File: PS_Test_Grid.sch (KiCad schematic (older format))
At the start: 50 parts, among them J1 CONN_01X03, J10 CONN_01X01, J2 CONN_01X01, J3 CONN_01X01, J4 CONN_01X01, J5 CONN_01X01, J6 CONN_01X03, J7 CONN_01X01, J8 CONN_01X01, J9 CONN_01X01, Q1 PhotoTransistor, U1 NOA1212, U2 MCP6001R, U3 MCP6001R

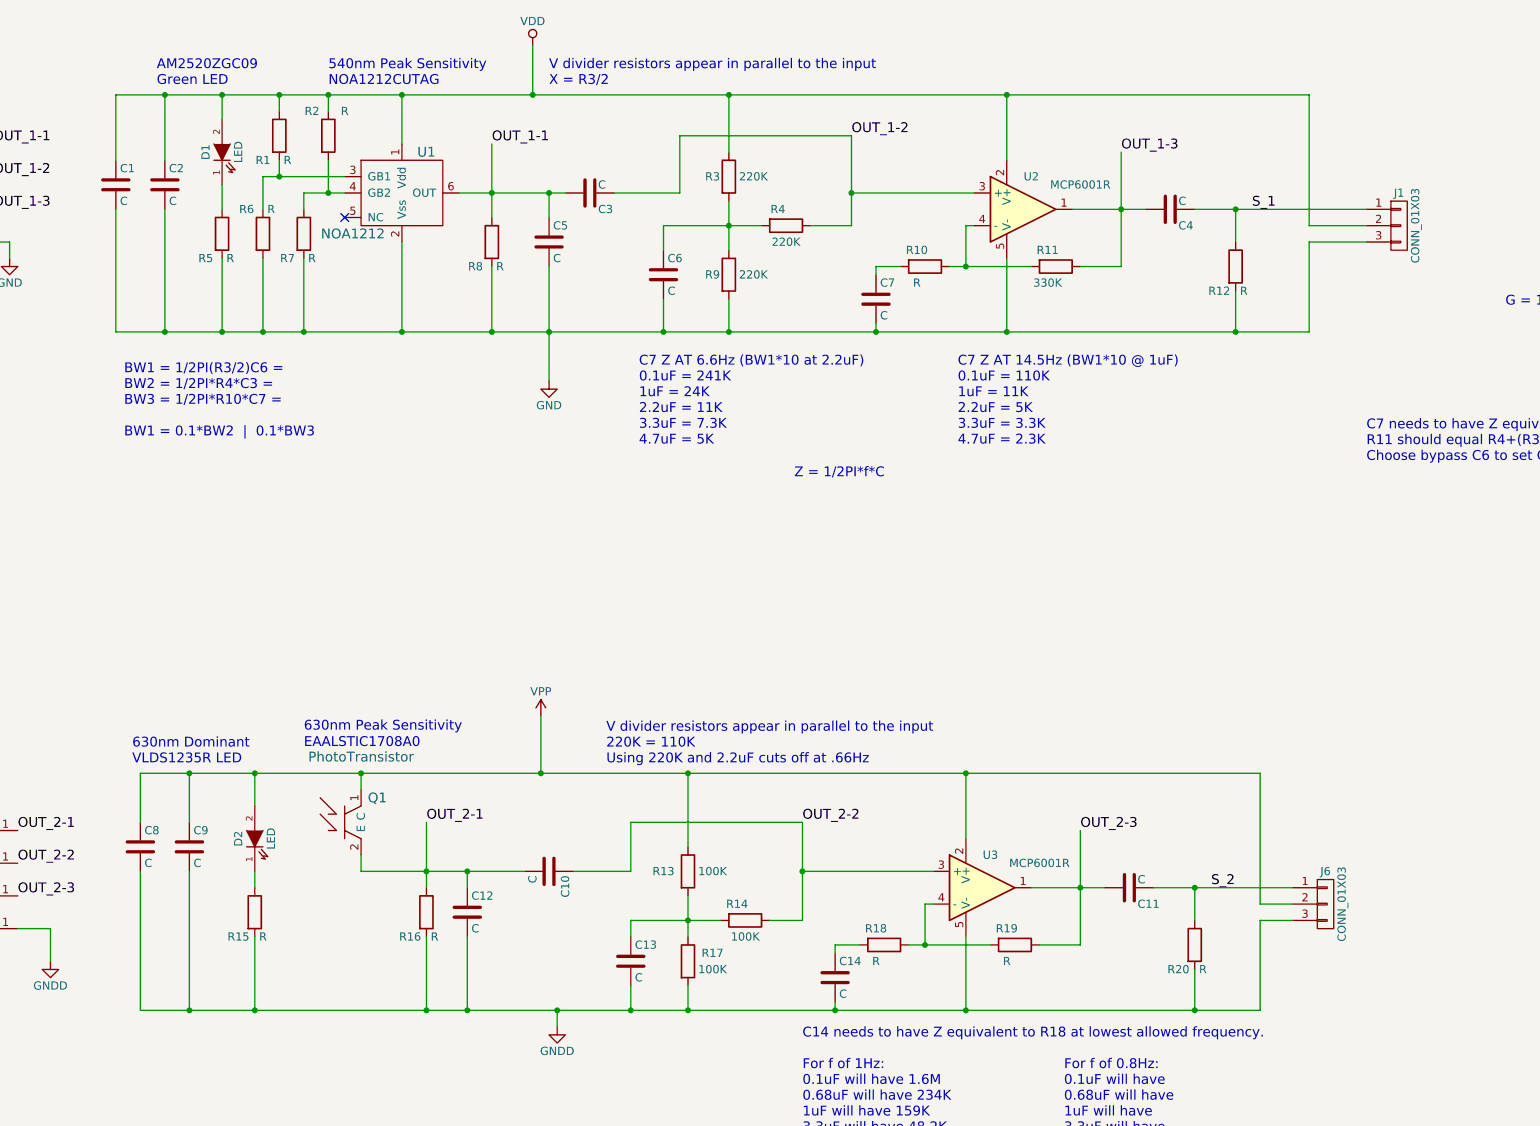
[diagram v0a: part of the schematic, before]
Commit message: saved notes
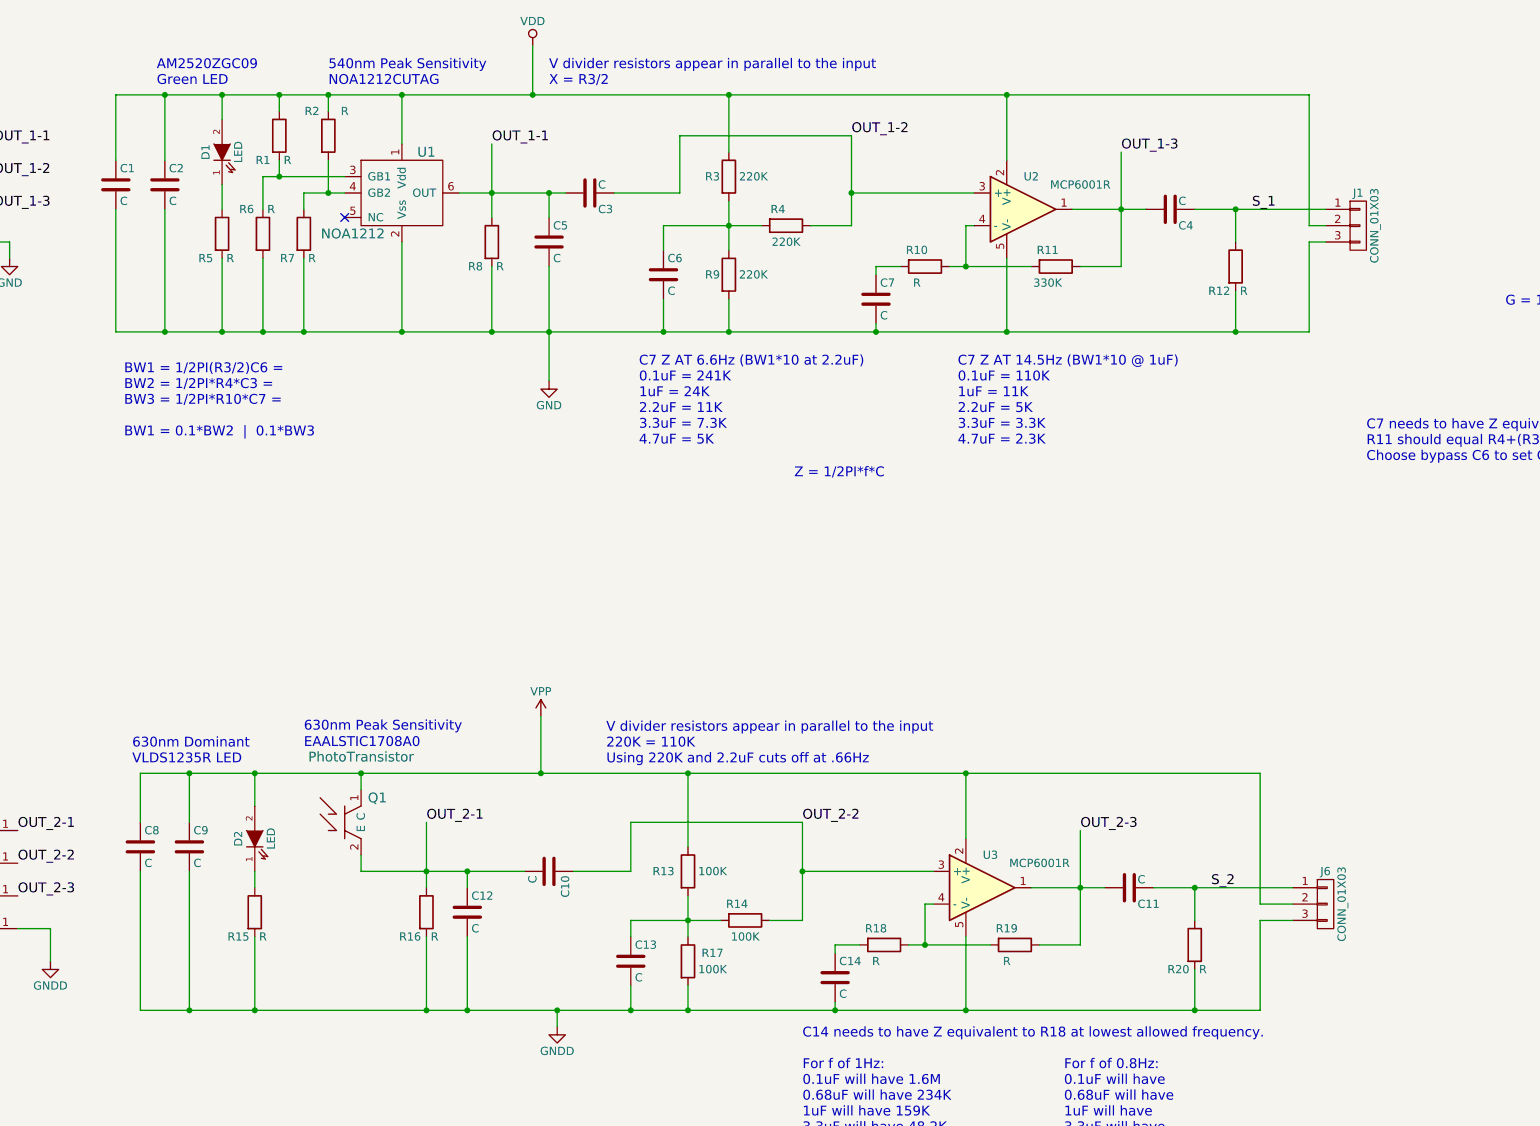
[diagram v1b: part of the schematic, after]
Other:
- moved on the sheet: J1
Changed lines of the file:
@@
 	7150 3550 7150 3000
 Wire Wire Line
-	8050 3150 8050 3850
+	8050 3150 8050 3550
+Wire Wire Line
+	8050 3550 8050 3850
 Wire Wire Line
 	10850 3550 10850 3100
@@
 	7150 2100 7150 2400
 Wire Wire Line
-	5400 2100 12700 2100
+	5400 2100 5700 2100
+Wire Wire Line
+	5700 2100 6050 2100
+Wire Wire Line
+	6050 2100 6400 2100
+Wire Wire Line
+	6400 2100 6700 2100
+Wire Wire Line
+	6700 2100 7150 2100
+Wire Wire Line
+	7150 2100 7950 2100
+Wire Wire Line
+	7950 2100 9150 2100
+Wire Wire Line
+	9150 2100 10850 2100
+Wire Wire Line
+	10850 2100 12700 2100
 Wire Wire Line
 	7950 2100 7950 1800
@@
 Connection ~ 7150 3550
 Wire Wire Line
-	7500 2700 8150 2700
-Wire Wire Line
-	7700 2400 7700 2850
+	7500 2700 7700 2700
+Wire Wire Line
+	7700 2700 8050 2700
+Wire Wire Line
+	8050 2700 8150 2700
+Wire Wire Line
+	7700 2400 7700 2700
+Wire Wire Line
+	7700 2700 7700 2850
 Wire Wire Line
 	7700 3550 7700 3150
@@
 Connection ~ 9150 2100
 Wire Wire Line
-	9150 2750 9150 3050
+	9150 2750 9150 2900
+Wire Wire Line
+	9150 2900 9150 3050
 Wire Wire Line
 	9150 3550 9150 3350
@@
 Connection ~ 9150 2900
 Wire Wire Line
-	11250 2800 11700 2800
-Wire Wire Line
-	11550 2450 11550 3150
+	11250 2800 11550 2800
+Wire Wire Line
+	11550 2800 11700 2800
+Wire Wire Line
+	11550 2450 11550 2800
+Wire Wire Line
+	11550 2800 11550 3150
 Wire Wire Line
 	11550 3150 11300 3150
@@
 	10600 2900 10600 3150
 Wire Wire Line
-	10500 3150 11000 3150
+	10500 3150 10600 3150
+Wire Wire Line
+	10600 3150 11000 3150
 Connection ~ 10600 3150
 Wire Wire Line
@@
 Connection ~ 6550 3550
 Wire Wire Line
-	6550 2700 6800 2700
+	6550 2700 6700 2700
+Wire Wire Line
+	6700 2700 6800 2700
 Wire Wire Line
 	6550 2700 6550 2800
@@
 Connection ~ 6700 2700
 Wire Wire Line
-	6300 2600 6800 2600
+	6300 2600 6400 2600
+Wire Wire Line
+	6400 2600 6800 2600
 Wire Wire Line
 	6300 2600 6300 2800
@@
 Connection ~ 7550 7700
 Wire Wire Line
-	6900 6850 7900 6850
+	6900 6850 7300 6850
+Wire Wire Line
+	7300 6850 7550 6850
+Wire Wire Line
+	7550 6850 7900 6850
 Wire Wire Line
 	7550 6850 7550 6950
@@
 Connection ~ 7550 6850
 Wire Wire Line
-	7300 6550 7300 6950
+	7300 6550 7300 6850
+Wire Wire Line
+	7300 6850 7300 6950
 Connection ~ 7300 6850
 Wire Wire Line
@@
 Connection ~ 11550 2800
 Wire Wire Line
-	12000 2800 13050 2800
+	12000 2800 12250 2800
+Wire Wire Line
+	12250 2800 12800 2800
 Wire Wire Line
 	12250 2800 12250 3000
@@
 Connection ~ 8900 6250
 Wire Wire Line
-	8900 7000 8900 7250
+	8900 7000 8900 7150
+Wire Wire Line
+	8900 7150 8900 7250
 Wire Wire Line
 	8900 7700 8900 7550
@@
 Connection ~ 8900 7150
 Wire Wire Line
-	11000 6950 11450 6950
-Wire Wire Line
-	11300 6600 11300 7300
+	11000 6950 11300 6950
+Wire Wire Line
+	11300 6950 11450 6950
+Wire Wire Line
+	11300 6600 11300 6950
+Wire Wire Line
+	11300 6950 11300 7300
 Wire Wire Line
 	11300 7300 11050 7300
@@
 	10350 7050 10350 7300
 Wire Wire Line
-	10250 7300 10750 7300
+	10250 7300 10350 7300
+Wire Wire Line
+	10350 7300 10750 7300
 Connection ~ 10350 7300
 Text Notes 8400 6200 0    60   ~ 0
@@
 Connection ~ 11300 6950
 Wire Wire Line
-	11750 6950 12600 6950
+	11750 6950 12000 6950
+Wire Wire Line
+	12000 6950 12600 6950
 Wire Wire Line
 	12000 6950 12000 7150
@@
 Connection ~ 5850 7700
 Wire Wire Line
-	5550 6250 12400 6250
-Wire Wire Line
-	5550 7700 12400 7700
+	5550 6250 5850 6250
+Wire Wire Line
+	5850 6250 6250 6250
+Wire Wire Line
+	6250 6250 6900 6250
+Wire Wire Line
+	6900 6250 8000 6250
+Wire Wire Line
+	8000 6250 8900 6250
+Wire Wire Line
+	8900 6250 10600 6250
+Wire Wire Line
+	10600 6250 12400 6250
+Wire Wire Line
+	5550 7700 5850 7700
+Wire Wire Line
+	5850 7700 6250 7700
+Wire Wire Line
+	6250 7700 7300 7700
+Wire Wire Line
+	7300 7700 7550 7700
+Wire Wire Line
+	7550 7700 8100 7700
+Wire Wire Line
+	8100 7700 8550 7700
+Wire Wire Line
+	8550 7700 8900 7700
+Wire Wire Line
+	8900 7700 9800 7700
+Wire Wire Line
+	9800 7700 10600 7700
+Wire Wire Line
+	10600 7700 12000 7700
+Wire Wire Line
+	12000 7700 12400 7700
 Connection ~ 10600 7700
 $Comp
@@
 L CONN_01X03 J1
 U 1 1 5B92B63C
-P 13250 2900
-F 0 "J1" H 13250 3100 50  0000 C CNN
-F 1 "CONN_01X03" V 13350 2900 50  0000 C CNN
-F 2 "Pin_Headers:Pin_Header_Straight_1x03_Pitch2.54mm" H 13250 2900 50  0001 C CNN
-F 3 "" H 13250 2900 50  0001 C CNN
-	1    13250 2900
+P 13000 2900
+F 0 "J1" H 13000 3100 50  0000 C CNN
+F 1 "CONN_01X03" V 13100 2900 50  0000 C CNN
+F 2 "Pin_Headers:Pin_Header_Straight_1x03_Pitch2.54mm" H 13000 2900 50  0001 C CNN
+F 3 "" H 13000 2900 50  0001 C CNN
+	1    13000 2900
 	1    0    0    -1
 $EndComp
@@
 	12400 6250 12400 7050
 Wire Wire Line
-	13050 2900 12700 2900
-Wire Wire Line
-	13050 3000 12700 3000
+	12800 2900 12700 2900
+Wire Wire Line
+	12800 3000 12700 3000
 Wire Wire Line
 	12700 3000 12700 3550
@@
 AM2520ZGC09\nGreen LED
 Wire Wire Line
-	12700 3550 5400 3550
+	12700 3550 12250 3550
+Wire Wire Line
+	12250 3550 10850 3550
+Wire Wire Line
+	10850 3550 10050 3550
+Wire Wire Line
+	10050 3550 9150 3550
+Wire Wire Line
+	9150 3550 8750 3550
+Wire Wire Line
+	8750 3550 8050 3550
+Wire Wire Line
+	8050 3550 7700 3550
+Wire Wire Line
+	7700 3550 7150 3550
+Wire Wire Line
+	7150 3550 6550 3550
+Wire Wire Line
+	6550 3550 6300 3550
+Wire Wire Line
+	6300 3550 6050 3550
+Wire Wire Line
+	6050 3550 5700 3550
+Wire Wire Line
+	5700 3550 5400 3550
 Wire Wire Line
 	10650 2700 9900 2700
 Wire Wire Line
-	9900 2350 9900 2900
+	9900 2350 9900 2700
+Wire Wire Line
+	9900 2700 9900 2900
 Wire Wire Line
 	9900 2900 9650 2900
 Wire Wire Line
-	8750 2900 9350 2900
+	8750 2900 9150 2900
+Wire Wire Line
+	9150 2900 9350 2900
 Wire Wire Line
 	8750 3050 8750 2900
@@
 	8550 6550 9600 6550
 Wire Wire Line
-	9600 6550 9600 7150
+	9600 6550 9600 6850
+Wire Wire Line
+	9600 6850 9600 7150
 Wire Wire Line
 	9600 6850 10400 6850
 Wire Wire Line
-	8550 7150 9100 7150
+	8550 7150 8900 7150
+Wire Wire Line
+	8900 7150 9100 7150
 Wire Wire Line
 	8550 7250 8550 7150
